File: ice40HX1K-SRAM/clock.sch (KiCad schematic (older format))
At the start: 2 parts

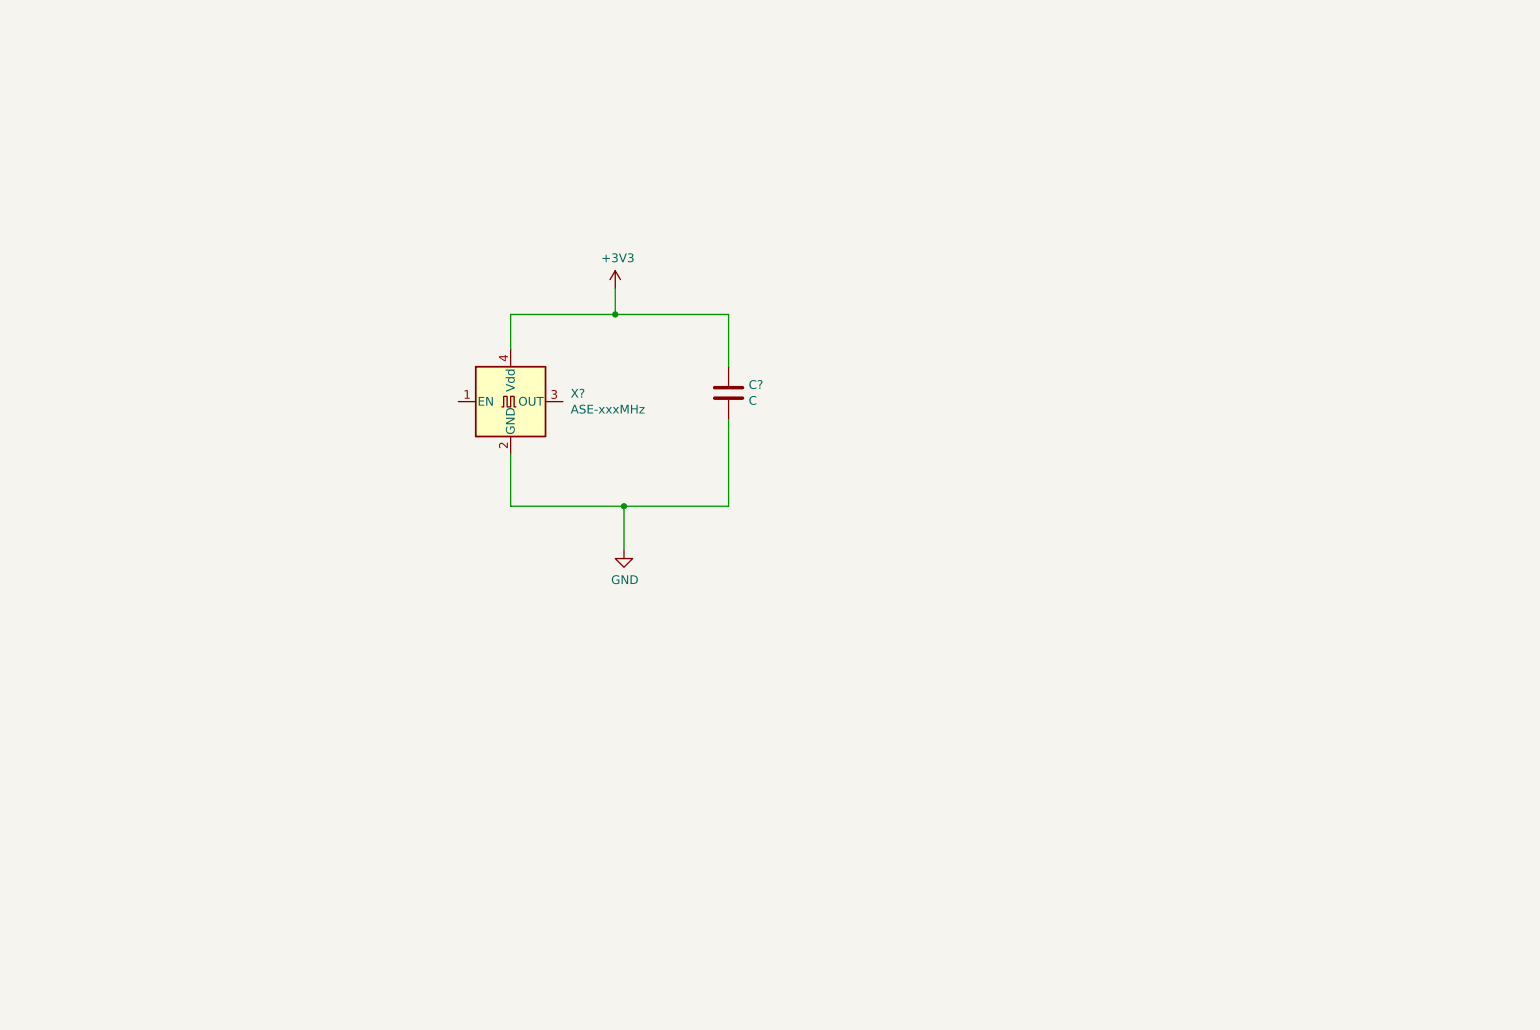
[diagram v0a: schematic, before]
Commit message: add  XTAL
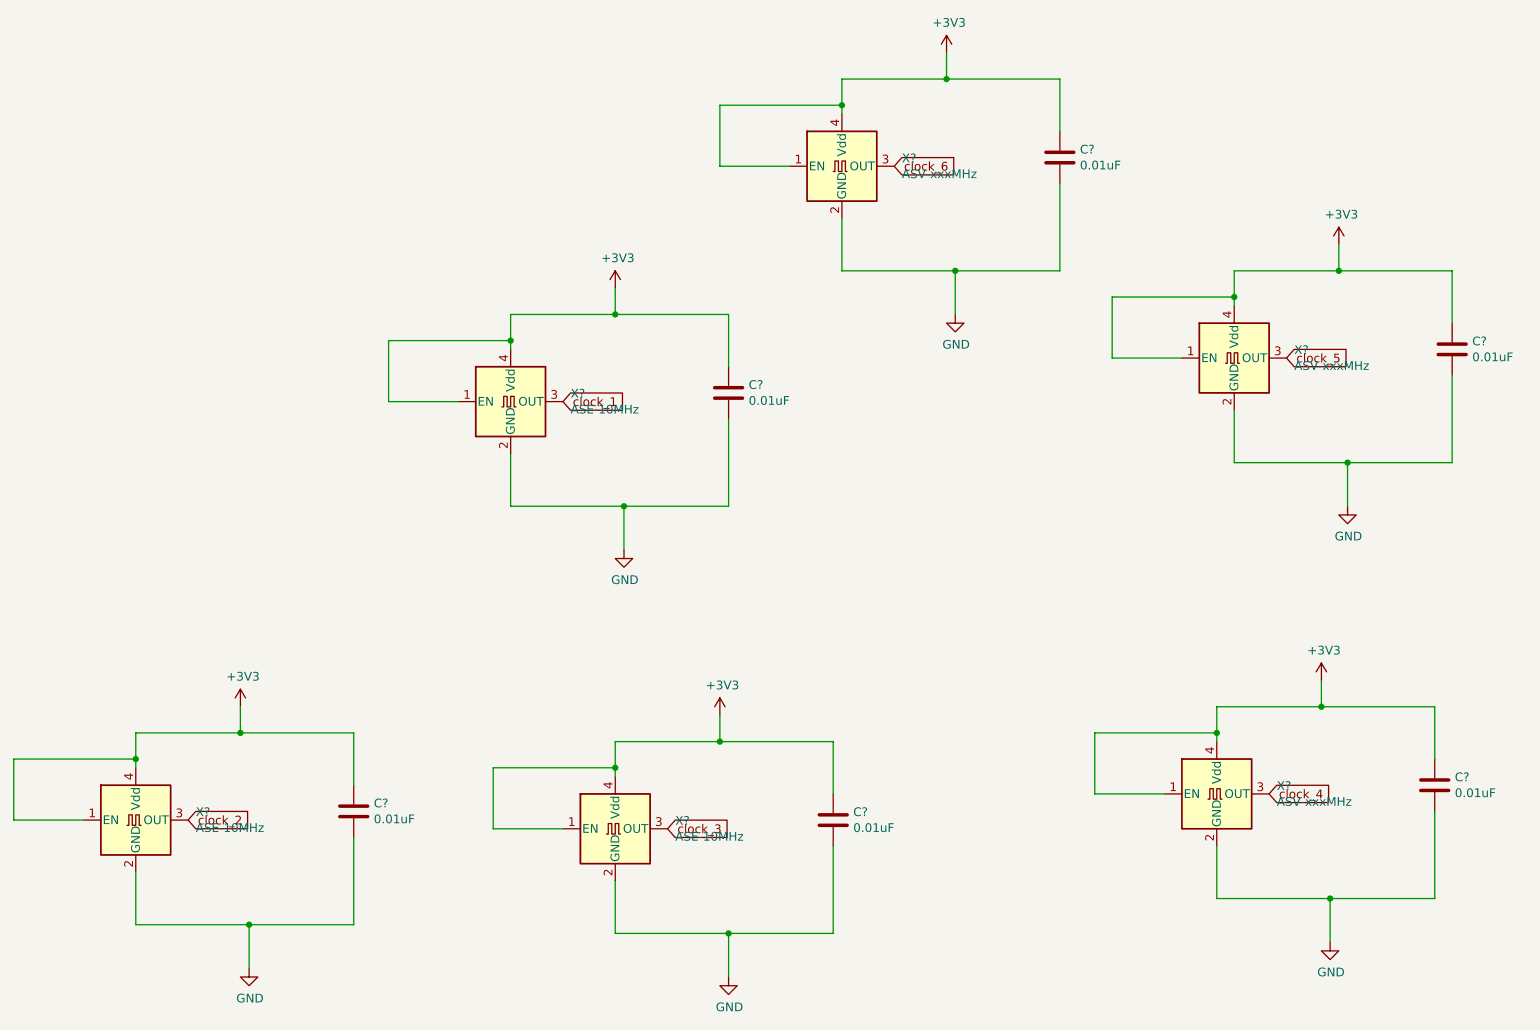
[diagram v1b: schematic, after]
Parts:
- added C? (x5): 0.01uF, symbol Device:C
- added X? (x3): ASV-xxxMHz, Oscillator:Oscillator_SMD_Abracon_ASV-4Pin_7.0x5.1mm, symbol Oscillator:ASV-xxxMHz
- added X? (x2): ASE-10MHz, Oscillator:Oscillator_SMD_Abracon_ASE-4Pin_3.2x2.5mm, symbol Oscillator:ASE-xxxMHz
- C?: value C -> 0.01uF
- X?: value ASE-xxxMHz -> ASE-10MHz
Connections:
- net +3V3: now also X?.1 (EN), C?.1, C?.1, C?.1, C?.1, C?.1, X?.1 (EN), X?.1 (EN), X?.1 (EN), X?.1 (EN), X?.1 (EN), X?.4 (Vdd), X?.4 (Vdd), X?.4 (Vdd), X?.4 (Vdd), X?.4 (Vdd)
- net GND: now also C?.2, C?.2, C?.2, C?.2, C?.2, X?.2 (GND), X?.2 (GND), X?.2 (GND), X?.2 (GND), X?.2 (GND)
- net clock_1: now reaches X?.3 (OUT)
- new net clock_2: X?.3 (OUT)
- new net clock_3: X?.3 (OUT)
- new net clock_4: X?.3 (OUT)
- new net clock_5: X?.3 (OUT)
- new net clock_6: X?.3 (OUT)
